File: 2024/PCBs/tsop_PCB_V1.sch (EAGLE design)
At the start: 38 parts, among them IC1 CD74HC4067SM96, IC2 CD74HC4067SM96, Q1 BSS138

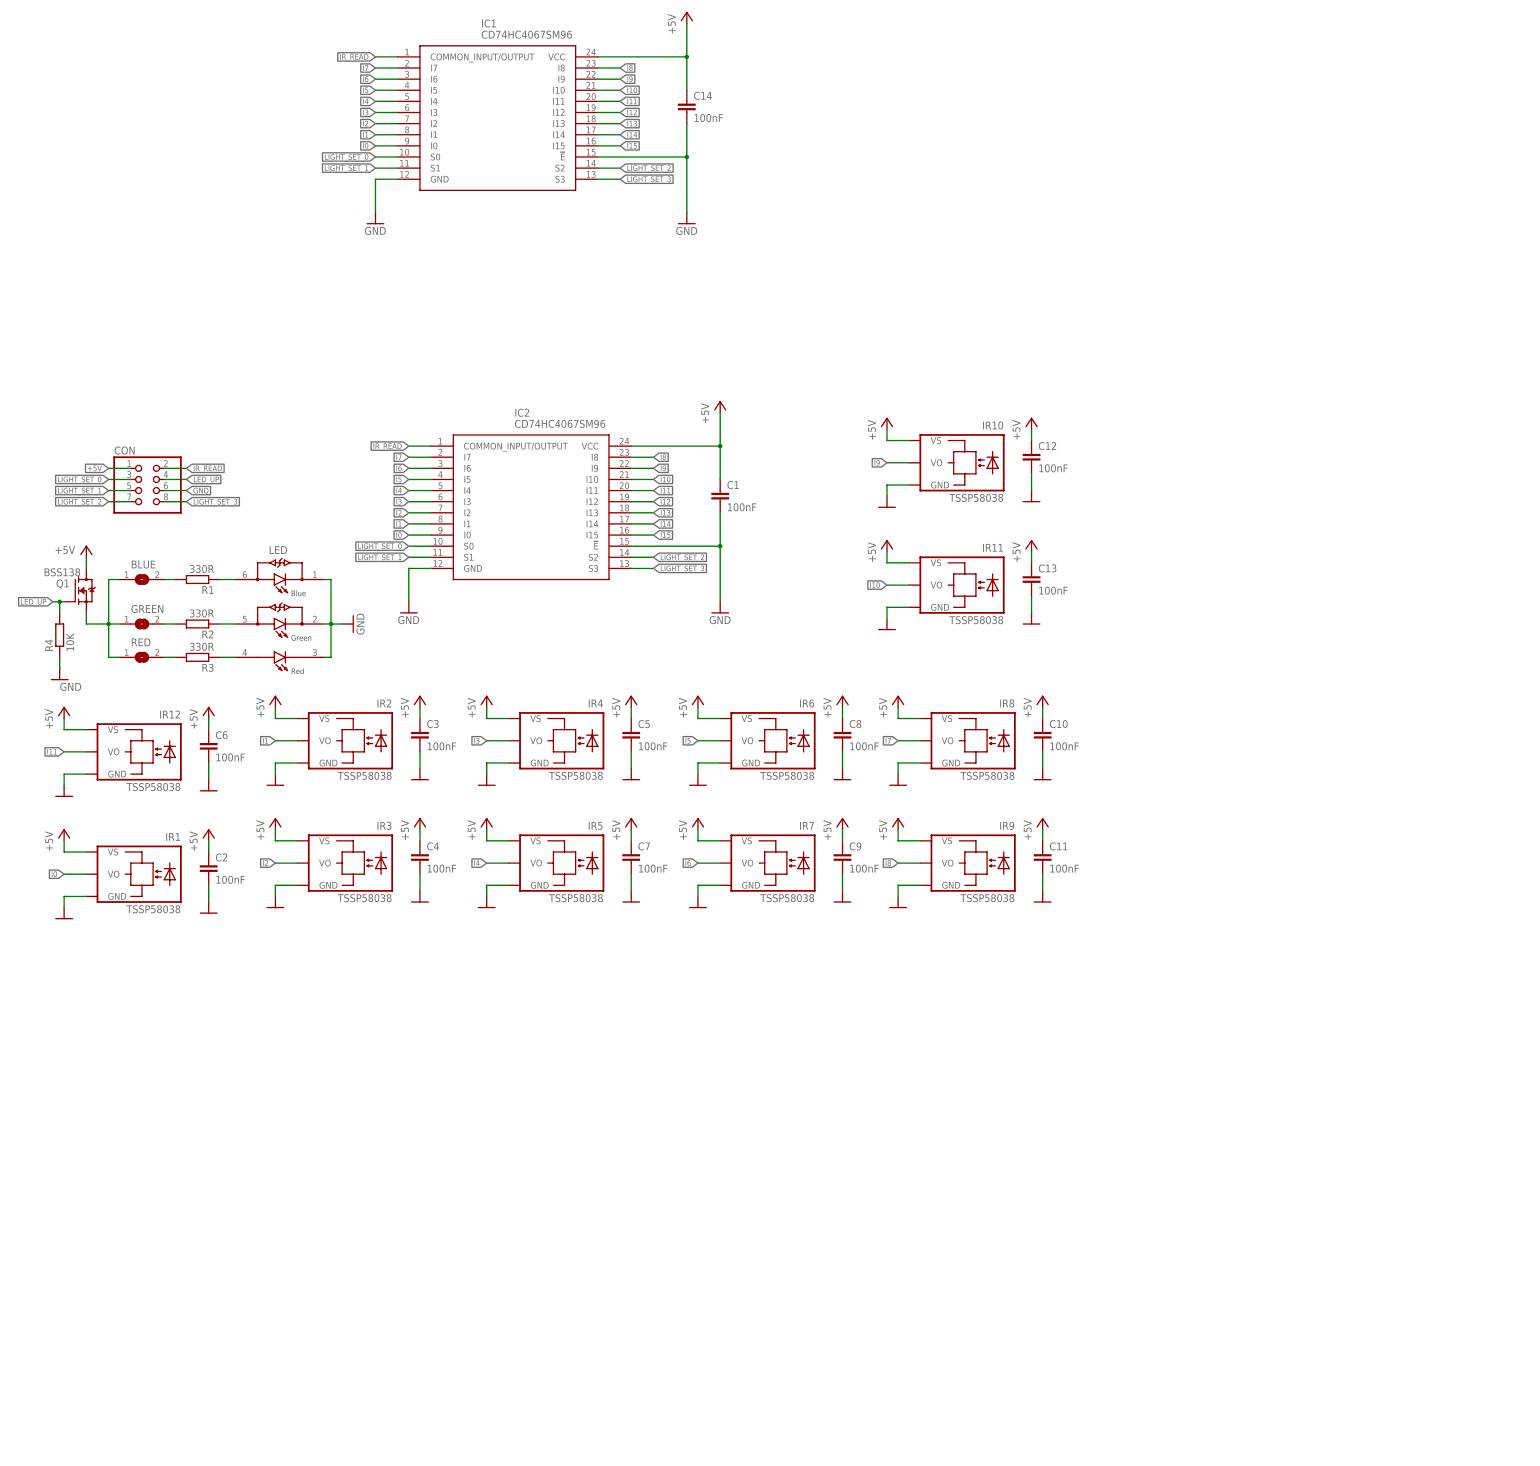
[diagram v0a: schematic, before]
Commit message: tsop
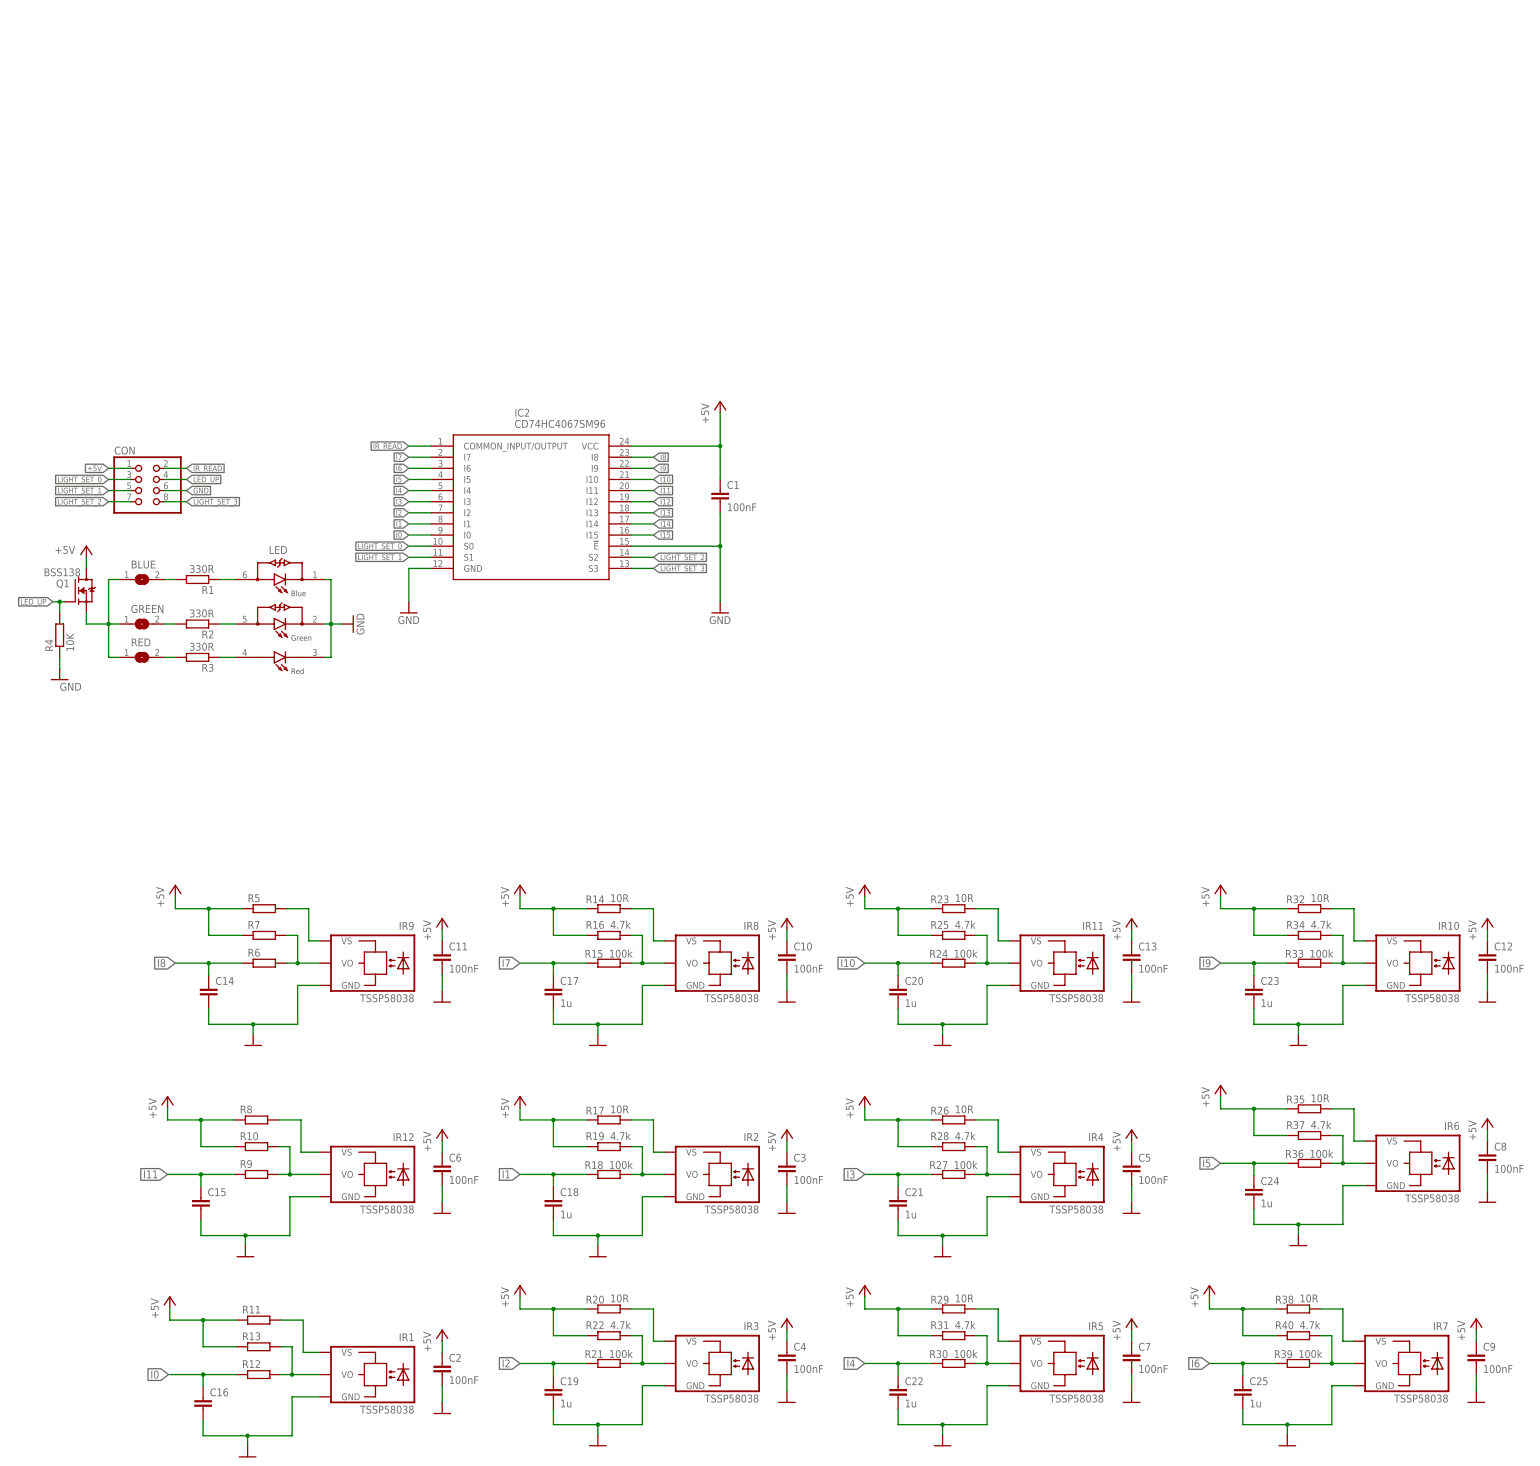
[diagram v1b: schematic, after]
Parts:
- removed IC1: CD74HC4067SM96, SamacSys_Parts:CD74HC4067SM96
- added C15, C16: (no value), rcl:C-EUC0805
- added C17, C18, C19, C20, C21, C22, C23, C24, C25: 1u, rcl:C-EUC0805
- added R10, R11, R12, R13, R5, R6, R7, R8, R9: (no value), rcl:R-EU_R0805
- added R14, R17, R20, R23, R26, R29, R32, R35, R38: 10R, rcl:R-EU_R0805
- added R15, R18, R21, R24, R27, R30, R33, R36, R39: 100k, rcl:R-EU_R0805
- added R16, R19, R22, R25, R28, R31, R34, R37, R40: 4.7k, rcl:R-EU_R0805
- C14: value 100nF -> (none)
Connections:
- new net N$10: IR8.VS, R14.2
- new net N$11: IR2.VS, R17.2
- new net N$12: IR3.VS, R20.2
- new net N$13: IR11.VS, R23.2
- new net N$14: IR4.VS, R26.2
- new net N$15: IR5.VS, R29.2
- new net N$16: IR10.VS, R32.2
- new net N$17: IR9.VS, R5.2
- new net N$18: IR6.VS, R35.2
- new net N$19: IR7.VS, R38.2
- new net N$20: IR12.VO, R10.2, R9.2
- new net N$21: IR9.VO, R6.2, R7.2
- new net N$22: IR5.VO, R30.2, R31.2
- new net N$23: IR1.VO, R12.2, R13.2
- new net N$25: IR8.VO, R15.2, R16.2
- new net N$26: IR4.VO, R27.2, R28.2
- new net N$27: IR2.VO, R18.2, R19.2
- new net N$29: IR11.VO, R24.2, R25.2
- new net N$30: IR3.VO, R21.2, R22.2
- new net N$32: IR10.VO, R33.2, R34.2
- new net N$34: IR6.VO, R36.2, R37.2
- new net N$36: IR7.VO, R39.2, R40.2
- new net N$8: IR12.VS, R8.2
- new net N$9: IR1.VS, R11.2
- net +5V: now also R10.1, R11.1, R13.1, R14.1, R16.1, R17.1, R19.1, R20.1, R22.1, R23.1, R25.1, R26.1, R28.1, R29.1, R31.1, R32.1, R34.1, R35.1, R37.1, R38.1, R40.1, R5.1, R7.1, R8.1; no longer C14.1, IC1.VCC, IR1.VS, IR10.VS, IR11.VS, IR12.VS, IR2.VS, IR3.VS, IR4.VS, IR5.VS, IR6.VS, IR7.VS, IR8.VS, IR9.VS
- net GND: now also C15.2, C16.2, C17.2, C18.2, C19.2, C20.2, C21.2, C22.2, C23.2, C24.2, C25.2; no longer IC1.!E, IC1.GND
- net I0: now also C16.1, R12.1; no longer IC1.I0, IR1.VO
- net I1: now also C18.1, R18.1; no longer IC1.I1, IR2.VO
- net I10: now also C20.1, R24.1; no longer IC1.I10, IR11.VO
- net I11: now also C15.1, R9.1; no longer IC1.I11, IR12.VO
- net I12: no longer IC1.I12
- net I13: no longer IC1.I13
- net I14: no longer IC1.I14
- net I15: no longer IC1.I15
- net I2: now also C19.1, R21.1; no longer IC1.I2, IR3.VO
- net I3: now also C21.1, R27.1; no longer IC1.I3, IR4.VO
- net I4: now also C22.1, R30.1; no longer IC1.I4, IR5.VO
- net I5: now also C24.1, R36.1; no longer IC1.I5, IR6.VO
- net I6: now also C25.1, R39.1; no longer IC1.I6, IR7.VO
- net I7: now also C17.1, R15.1; no longer IC1.I7, IR8.VO
- net I8: now also C14.1, R6.1; no longer IC1.I8, IR9.VO
- net I9: now also C23.1, R33.1; no longer IC1.I9, IR10.VO
- net IR_READ: no longer IC1.COMMON_INPUT/OUTPUT
- net LIGHT_SET_0: no longer IC1.S0
- net LIGHT_SET_1: no longer IC1.S1
- net LIGHT_SET_2: no longer IC1.S2
- net LIGHT_SET_3: no longer IC1.S3
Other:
- moved on the sheet: C10, C11, C12, C13, C14, C2, C3, C4, C5, C6, C7, C8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
